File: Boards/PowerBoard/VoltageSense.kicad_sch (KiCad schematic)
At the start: 40 parts

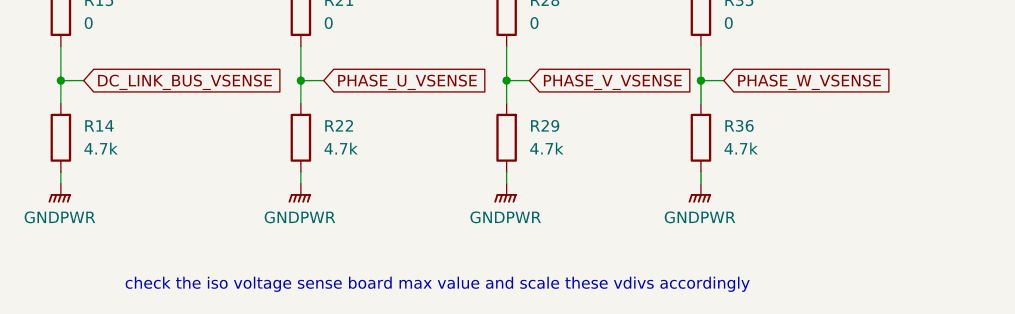
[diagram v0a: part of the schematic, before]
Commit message: Update Layouts
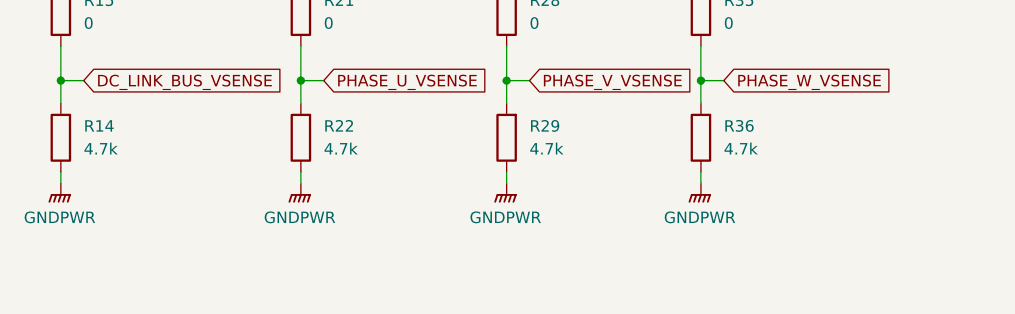
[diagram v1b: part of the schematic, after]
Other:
- note removed: "check the iso voltage sense board max value and scale these vdivs accordingly"
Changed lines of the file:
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@@
 	(generator_version "9.0")
 	(paper "A4")
-	(text "check the iso voltage sense board max value and scale these vdivs accordingly"
-		(exclude_from_sim no)
-		(at 59.6268 106.5937 0)
-		(effects
-			(font
-				(size 1.27 1.27)
-			)
-		)
-	)
 	(junction
 		(at 158.75 55.88)
